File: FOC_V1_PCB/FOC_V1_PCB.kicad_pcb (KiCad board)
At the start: 4 copper layers, 72.6 x 72.6 mm, 95 parts, among them J1 ST-Link_01x05, J10 C, J2 Enc_MCU_01x06, J4 CAN_01x04, J6 +V, J7 GND, J8 A, J9 B, SW1 TS-1002S-05026C, U1 STM32F405RGT6, U10 TJA1051T/3/1J, U11 ME6211, U2 DRV8301DCAR, U3 IRFS7530TRL7PP, U4 IRFS7530TRL7PP, U5 IRFS7530TRL7PP, U6 IRFS7530TRL7PP, U7 IRFS7530TRL7PP, U8 IRFS7530TRL7PP, Y1 Crystal_GND24

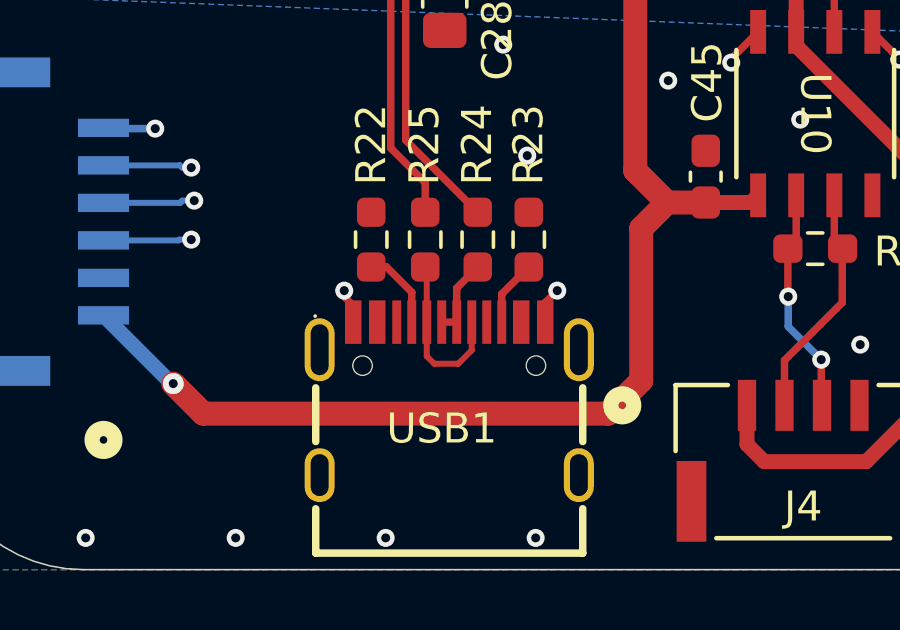
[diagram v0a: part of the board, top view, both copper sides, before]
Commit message: new V1.3 design (fixed USB-C)
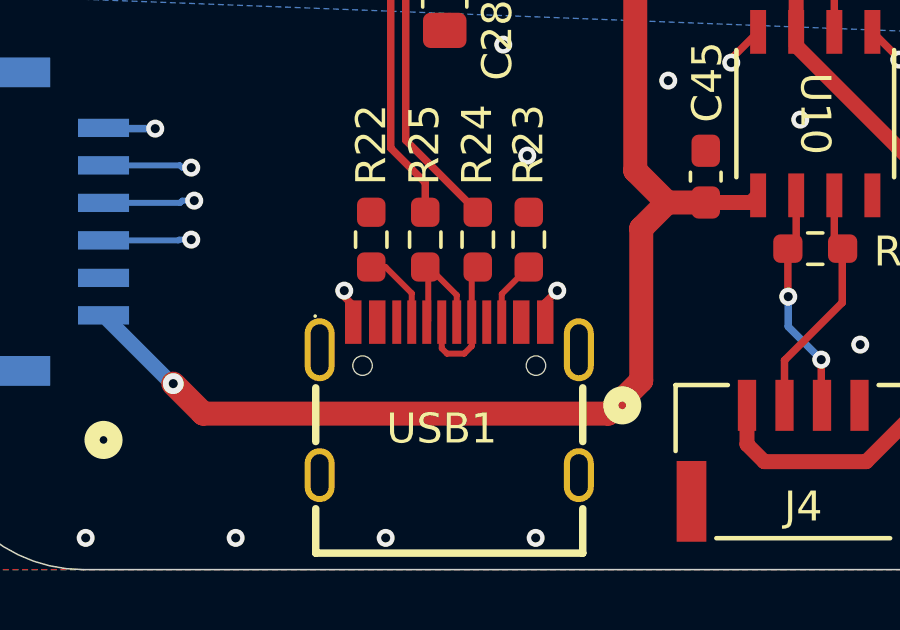
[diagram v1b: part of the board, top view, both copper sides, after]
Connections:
- R24 pad 1: Net-(USB1-DN1) -> Net-(USB1-DP1)
- R25 pad 1: Net-(USB1-DN2) -> Net-(USB1-DN1)
- USB1 pad A6: Net-(USB1-DN1) -> Net-(USB1-DP1)
- USB1 pad B6: Net-(USB1-DN2) -> Net-(USB1-DP1)
- USB1 pad B7: Net-(USB1-DN2) -> Net-(USB1-DN1)
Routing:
- net Net-(USB1-DN2): track 5.72 -> 0.00 mm
- net Net-(USB1-DP1): track 0.00 -> 4.77 mm
- net Net-(USB1-DN1): track 2.63 -> 4.24 mm
